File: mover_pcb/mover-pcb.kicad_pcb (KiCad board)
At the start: 2 copper layers, 47 x 62.5 mm, 10 parts, among them J1 Conn_01x03_Pin, J2 Conn_01x05_Pin, J3 Conn_01x05_Pin, J4 Conn_01x06_Pin, J5 Conn_01x04_Pin, J6 Conn_01x03_Pin

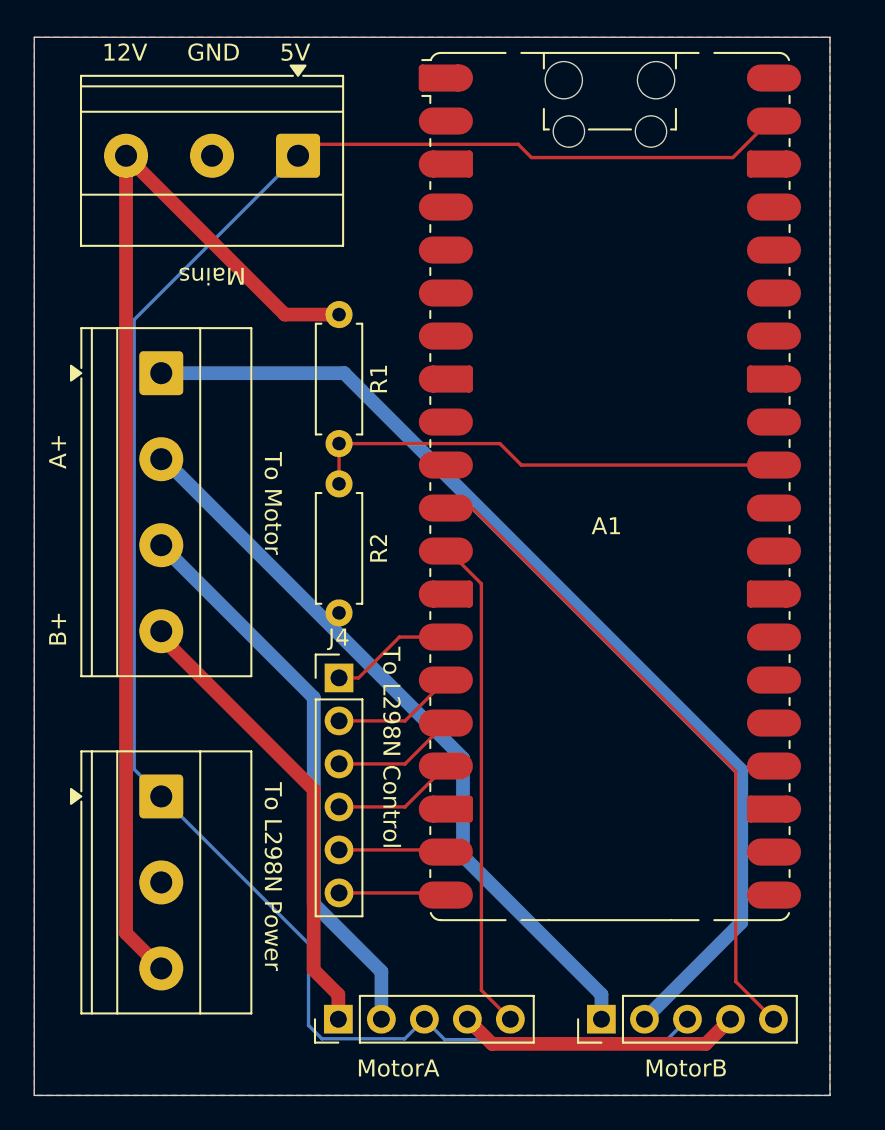
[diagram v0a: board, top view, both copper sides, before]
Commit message: update pcb; progress on controller
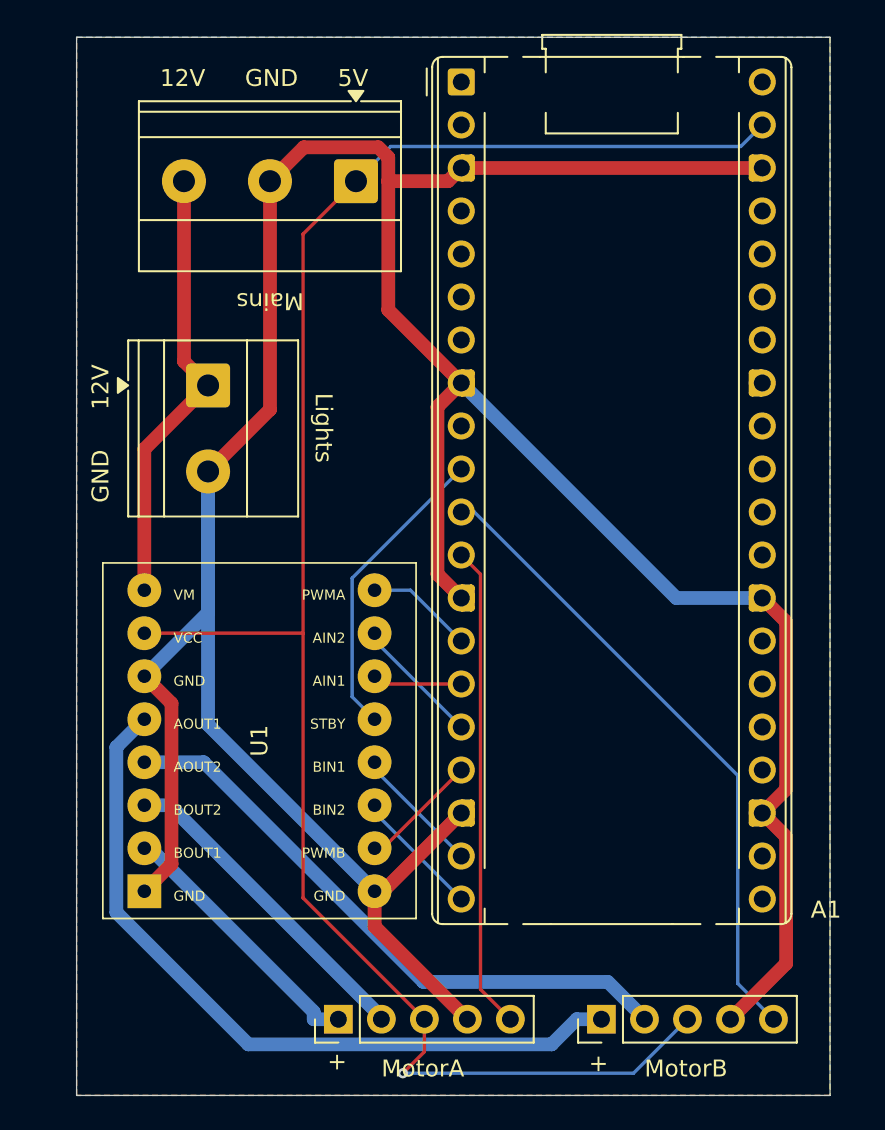
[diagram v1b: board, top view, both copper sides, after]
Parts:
- removed J5: Conn_01x04_Pin, TerminalBlock_Phoenix:TerminalBlock_Phoenix_MKDS-1,5-4-5.08_1x04_P5.08mm_Horizontal
- removed J6: Conn_01x03_Pin, TerminalBlock_Phoenix:TerminalBlock_Phoenix_MKDS-1,5-3-5.08_1x03_P5.08mm_Horizontal
- removed R1: 47k, Resistor_THT:R_Axial_DIN0207_L6.3mm_D2.5mm_P7.62mm_Horizontal
- removed R2: 10k, Resistor_THT:R_Axial_DIN0207_L6.3mm_D2.5mm_P7.62mm_Horizontal
- added U1: TB6612FNG, TB6612:TB6612FNG_Module, F.Cu at (110.3, 123.0)
- A1: footprint Module:RaspberryPi_Pico_Common_SMD -> Module:RaspberryPi_Pico_Common_THT
- J4: value Conn_01x06_Pin -> Conn_01x02_Pin; footprint Connector_PinHeader_2.54mm:PinHeader_1x06_P2.54mm_Vertical -> TerminalBlock_Phoenix:TerminalBlock_Phoenix_MKDS-1,5-2-5.08_1x02_P5.08mm_Horizontal
- moved A1 25.5 mm to (122.2, 84.1)
- moved J4 18.9 mm to (107.3, 102.1), turned to -90 degrees
- moved G*** 8.73 mm to (131.5, 103.0), turned to -90 degrees
- moved J1 3.73 mm to (116.0, 90.0)
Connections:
- A1 pad 10: unconnected-(A1-GPIO7-Pad10) -> Enable
- A1 pad 14: EnA -> PWMA
- A1 pad 17: EnB -> PWMB
- A1 pad 31: Voltage -> unconnected-(A1-GPIO26_ADC0-Pad31)
- J4 pad 1: EnA -> 12V
- J4 pad 2: IN1 -> GND
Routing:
- net GND: track 16.7 -> 202.6 mm
- net 12V: track 65.3 -> 26.3 mm
- net Voltage: track 28.6 -> 0.00 mm
- net MotorA-: track 61.0 -> 35.9 mm
- net Enable: track 0.00 -> 18.0 mm
- net MotorB-: track 33.4 -> 19.3 mm
- net MotorB+: track 27.3 -> 15.9 mm
- net EnA: track 7.31 -> 0.00 mm
- net EnB: track 7.31 -> 0.00 mm
- net PWMB: track 0.00 -> 7.03 mm
- net PWMA: track 0.00 -> 6.36 mm
- net 5V: track 113.4 -> 110.4 mm, vias 0 -> 1
- net IN1: track 7.31 -> 5.31 mm
- net IN3: track 6.36 -> 7.66 mm
- net IN4: track 6.36 -> 7.66 mm
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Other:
- board size 47 x 62.5 mm -> 44.5 x 62.5 mm
- board text added: "+"
- board text added: "Lights"
- board text removed: "A+"
- board text removed: "B+"
- board text removed: "To L298N Control"
- board text removed: "To L298N Power"
- board text removed: "To Motor"
